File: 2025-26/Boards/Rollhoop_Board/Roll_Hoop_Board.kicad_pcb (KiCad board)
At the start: 2 copper layers, 106.7 x 36 mm, 30 parts, among them J1 DTM13-12PA, J2 DTM13-12PA, J3 Conn_01x04_Pin, Q1 AO3401A, Q2 AO3400A, Q3 AO3400A, Q4 AO3400A, U2 SN65HVD230, U3 STM32C011F4Px, U4 UA78M33QDCYRQ1

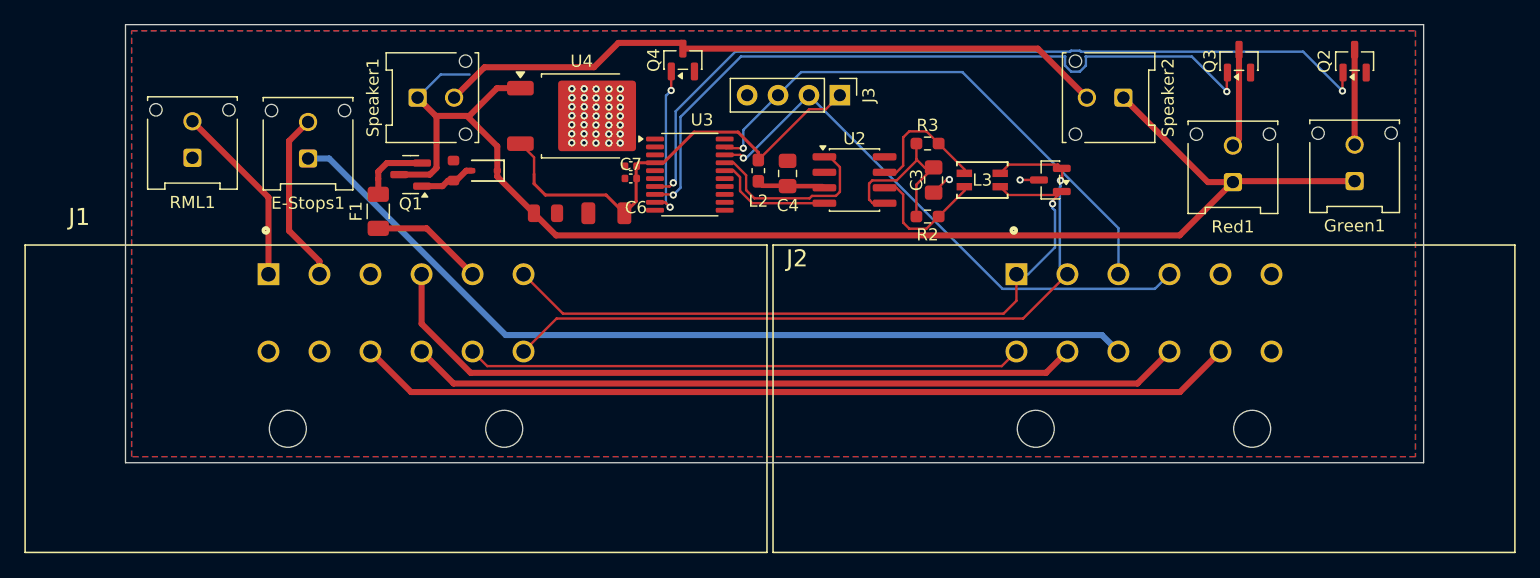
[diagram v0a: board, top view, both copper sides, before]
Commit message: Rollhoop board edit
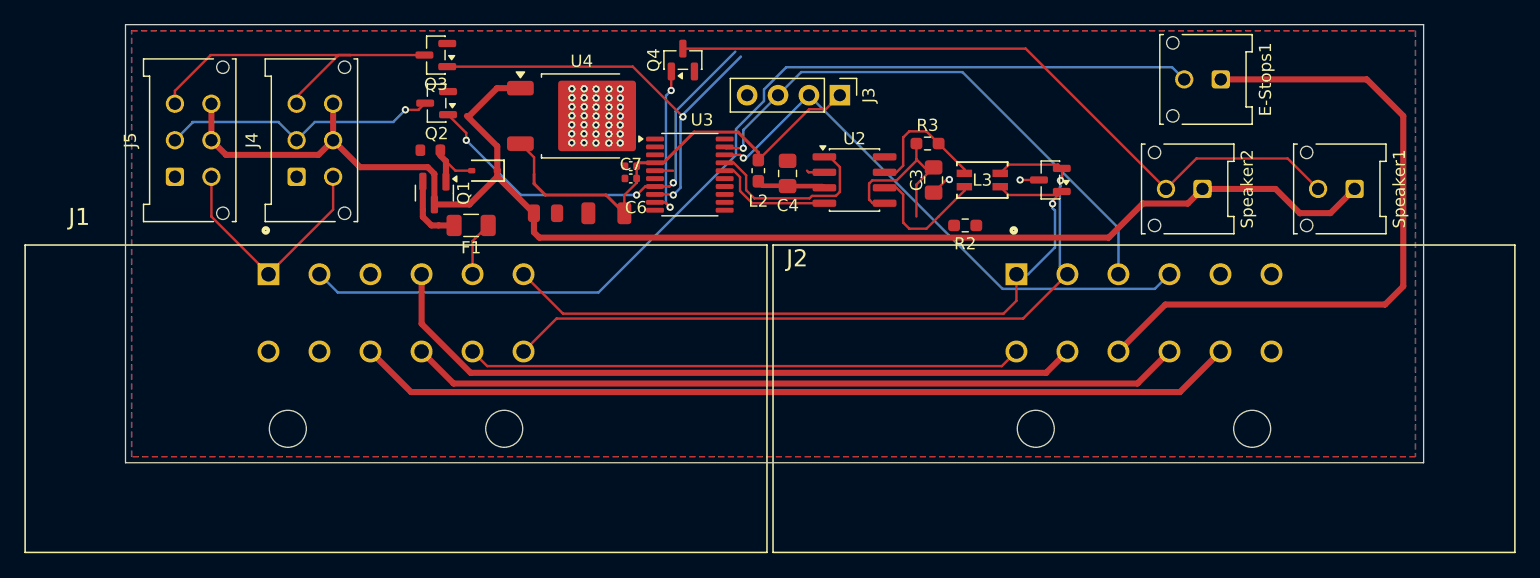
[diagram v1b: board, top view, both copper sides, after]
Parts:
- removed Green1, RML1, Red1: 043045-0212, Connector_Molex:Molex_Micro-Fit_3.0_43045-0212_2x01_P3.00mm_Vertical
- added J4: 043045-0612, Connector_Molex:Molex_Micro-Fit_3.0_43045-0612_2x03_P3.00mm_Vertical, F.Cu at (130.1, 37.5)
- added J5: 043045-0612, Connector_Molex:Molex_Micro-Fit_3.0_43045-0612_2x03_P3.00mm_Vertical, F.Cu at (120.1, 37.5)
- E-Stops1: value 043045-0212 -> 043045-0612
- moved Speaker1 77.4 mm to (217.0, 38.5), turned to -90 degrees
- moved Q2 75.5 mm to (141.6, 31.4), turned to 180 degrees
- moved E-Stops1 75.3 mm to (206.0, 29.5), turned to -90 degrees
- moved Q3 66.0 mm to (141.5, 27.5), turned to 180 degrees
- moved Speaker2 9.92 mm to (204.5, 38.5)
- moved F1 7.72 mm to (144.4, 41.5), turned to 180 degrees
- moved R2 3.18 mm to (185.0, 41.5)
- moved R1 2.53 mm to (141.1, 35.3), turned to 0 degrees
- moved Q1 2.47 mm to (141.4, 38.8), turned to -90 degrees
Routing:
- net RLH_SDC_IN: track 14.2 -> 81.6 mm
- net Green_LED: track 67.3 -> 34.9 mm, vias 2 -> 3
- net Red_LED: track 59.9 -> 36.3 mm
- net Red_Out: track 8.08 -> 29.2 mm
- net DSH_SDC_IN: track 73.9 -> 55.9 mm
- net Green_Out: track 7.80 -> 23.1 mm, vias 0 -> 1
- net +12V: track 116.1 -> 123.0 mm
- net RLH_RML_YELLOW: track 15.2 -> 20.2 mm
- net RLH_PWR: track 9.31 -> 4.54 mm
- net Speaker_Out: track 55.5 -> 59.0 mm
- net GND: track 3.31 -> 6.28 mm
- net Net-(Q1-G): track 4.61 -> 5.44 mm
